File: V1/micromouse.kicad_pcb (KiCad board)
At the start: 2 copper layers, 98.1 x 98.9 mm, 22 parts, among them J1 XT60-M, SW1 SW_SPST, SW2 SW_Push, SW3 SW_SPDT_312, SW4 SW_Push, U1 BUCK, U10 UART, U2 STM32 Blackpill, U3 N20 encoder right, U4 N20 encoder left, U5 TB6612FNG, U6 VL6180X, U7 VL6180X, U8 VL6180X

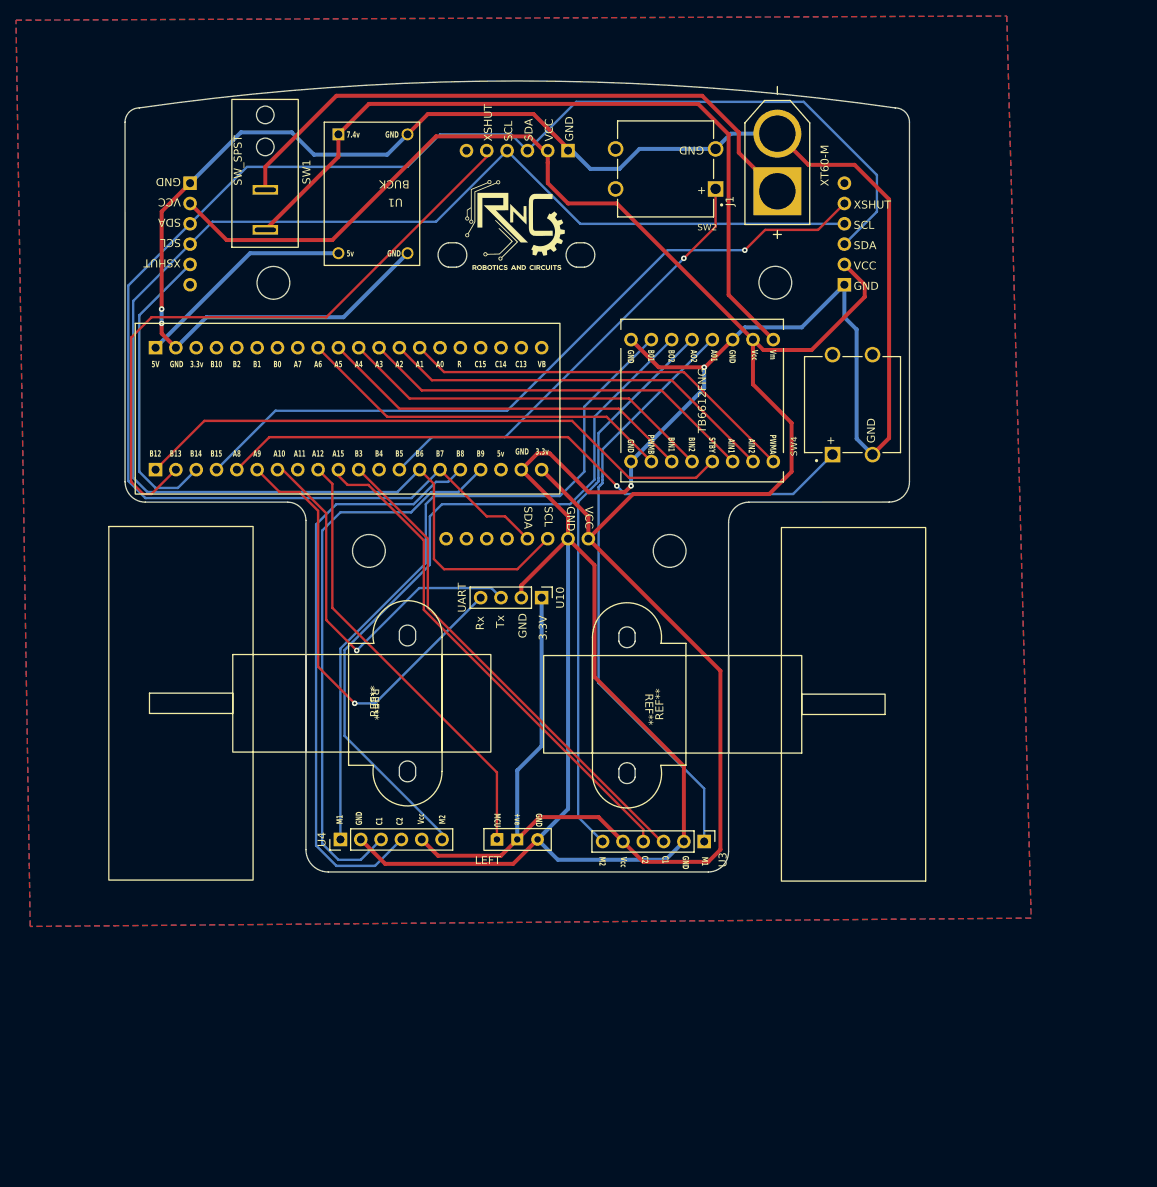
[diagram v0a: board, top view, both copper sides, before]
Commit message: v3 addition
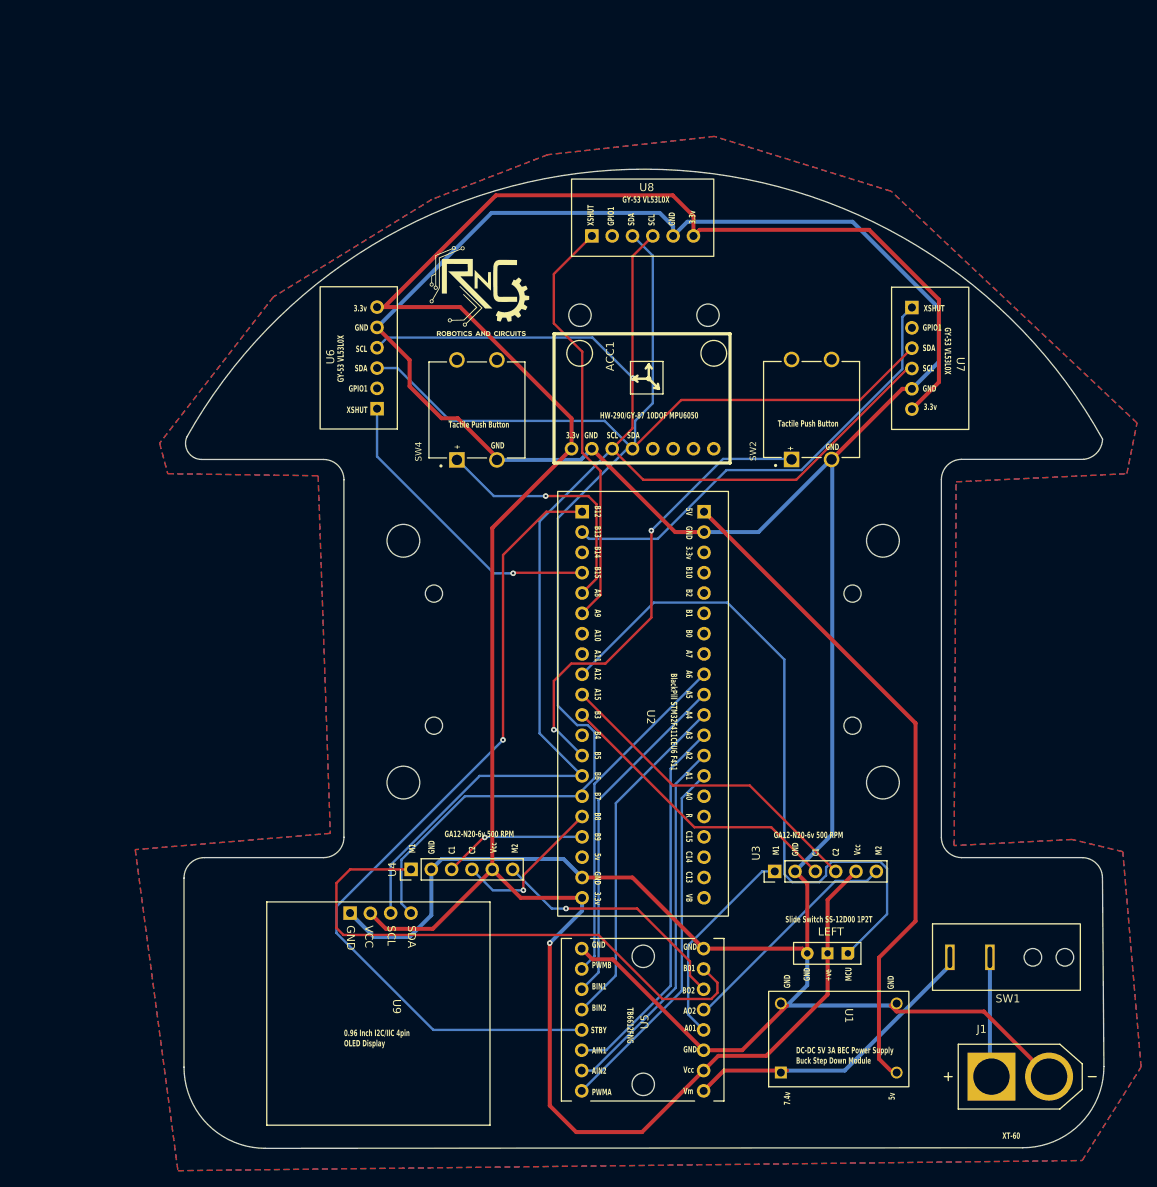
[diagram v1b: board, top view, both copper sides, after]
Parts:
- removed the G*** at (134.1, 40.9)
- removed the G*** at (134.1, 99.9)
- removed REF** (x2): n20 motor, n20 motor:n20 motor
- removed REF** (x2): n20 bracket, n20-bracket:Untitled
- removed REF**: castor, castor:castor
- removed U10: UART, Connector_PinHeader_2.54mm:PinHeader_1x04_P2.54mm_Vertical
- added G***: LOGO, rnc:rnc3, F.Cu at (129.7, 49.1)
- added U9: oled i2c, oled:oled, F.Cu at (118.5, 138.0)
- ACC1: moved to F.Cu
- U6: value VL6180X -> VL53L0X left; footprint VL6180X:VL6180X -> VL53L0X:VL53L0X; moved to F.Cu
- U7: value VL6180X -> VL53L0X right; footprint VL6180X:VL6180X -> VL53L0X:VL53L0X; moved to F.Cu
- U8: value VL6180X -> VL53L0X middle; footprint VL6180X:VL6180X -> VL53L0X:VL53L0X; moved to F.Cu
- moved SW1 135.0 mm to (195.4, 131.8), turned to 0 degrees
- moved U1 120.2 mm to (171.4, 140.6), turned to 90 degrees
- moved J1 118.2 mm to (197.0, 146.7), turned to 0 degrees
- moved U5 77.8 mm to (149.8, 139.6), turned to 180 degrees
- moved U6 55.8 mm to (119.1, 65.8)
- moved U7 48.2 mm to (180.9, 48.1), turned to -90 degrees
- moved SW4 47.0 mm to (129.1, 63.4)
- moved U8 42.1 mm to (140.9, 44.2), turned to 0 degrees
- moved SW3 39.7 mm to (173.0, 128.2), turned to 180 degrees
- moved ACC1 39.2 mm to (160.7, 70.0)
- moved SW2 35.2 mm to (170.9, 63.3), turned to 90 degrees
- moved U2 28.2 mm to (139.2, 73.6), turned to -90 degrees
- moved U3 9.58 mm to (166.3, 121.1), turned to 90 degrees
- moved U4 9.58 mm to (120.8, 120.8)
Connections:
- U2 pad 3: XSHUT 2 -> unconnected-(U2-B14-Pad3)
- U2 pad 6: Tx -> XSHUT 2
- U2 pad 7: Rx -> unconnected-(U2-A10-Pad7)
- U6 pad 1: unconnected-(U6-GPIO1-Pad1) -> 3.3v
- U6 pad 2: XSHUT 3 -> GND
- U6 pad 5: 3.3v -> unconnected-(U6-GPIO1-Pad5)
- U6 pad 6: GND -> XSHUT 3
- U7 pad 1: unconnected-(U7-GPIO1-Pad1) -> 3.3v
- U7 pad 2: XSHUT 1 -> GND
- U7 pad 5: 3.3v -> unconnected-(U7-GPIO1-Pad5)
- U7 pad 6: GND -> XSHUT 1
- U8 pad 1: unconnected-(U8-GPIO1-Pad1) -> 3.3v
- U8 pad 2: XSHUT 2 -> GND
- U8 pad 5: 3.3v -> unconnected-(U8-GPIO1-Pad5)
- U8 pad 6: GND -> XSHUT 2
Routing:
- net BO2: track 93.8 -> 31.1 mm, vias 0 -> 1
- net 7.4v: track 77.0 -> 15.0 mm
- net 7.4vb: track 95.6 -> 38.3 mm
- net Tx: track 56.9 -> 0.00 mm, vias 1 -> 0
- net 5v: track 27.8 -> 83.3 mm
- net XSHUT 3: track 92.3 -> 37.7 mm
- net encoder B2: track 74.1 -> 19.8 mm, vias 0 -> 1
- net encoder A2: track 71.3 -> 18.0 mm, vias 0 -> 1
- net push button: track 81.1 -> 31.5 mm
- net Rx: track 48.8 -> 0.00 mm, vias 1 -> 0
- net AO1: track 74.1 -> 26.0 mm
- net AO2: track 69.9 -> 28.7 mm
- net GND: track 430.2 -> 395.0 mm, vias 4 -> 0
- net slide_SW: track 55.5 -> 86.6 mm
- net STBY: track 75.9 -> 103.7 mm, vias 0 -> 1
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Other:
- board size 98.1 x 98.9 mm -> 115 x 122.4 mm
- board text added: "+"
- board text added: "+ve"
- board text added: "0.96 Inch I2C/IIC 4pin OLED Display"
- board text added: "3.3v"
- board text added: "5V"
- board text added: "5v"
- board text added: "7.4v"
- board text added: "A0"
- board text added: "A01"
- board text added: "A1"
- board text added: "A10"
- board text added: "A11"
- board text added: "A12"
- board text added: "A15"
- board text added: "A2"
- board text added: "A3"
- board text added: "A4"
- board text added: "A5"
- board text added: "A6"
- board text added: "A7"
- board text added: "A8"
- board text added: "A9"
- board text added: "AIN1"
- board text added: "AIN2"
- board text added: "AO2"
- board text added: "B0"
- board text added: "B01"
- board text added: "B1"
- board text added: "B10"
- board text added: "B12"
- board text added: "B13"
- board text added: "B14"
- board text added: "B15"
- board text added: "B2"
- board text added: "B3"
- board text added: "B4"
- board text added: "B5"
- board text added: "B6"
- board text added: "B7"
- board text added: "B8"
- board text added: "B9"
- board text added: "BIN1"
- board text added: "BIN2"
- board text added: "BO2"
- board text added: "BlackPill STM32F411CEU6 F411"
- board text added: "C1"
- board text added: "C13"
- board text added: "C14"
- board text added: "C15"
- board text added: "C2"
- board text added: "DC-DC 5V 3A BEC Power Supply Buck Step Down Module"
- board text added: "GA12-N20-6v 500 RPM"
- board text added: "GPIO1"
- board text added: "GY-53 VL53L0X"
- board text added: "HW-290/GY-87 10DOF MPU6050"
- board text added: "M1"
- board text added: "M2"
- board text added: "MCU"
- board text added: "PWMA"
- board text added: "PWMB"
- board text added: "R"
- board text added: "SCL"
- board text added: "SDA"
- board text added: "STBY"
- board text added: "Slide Switch SS-12D00 1P2T"
- board text added: "TB6612FNG"
- board text added: "Tactile Push Button"
- board text added: "VB"
- board text added: "Vcc"
- board text added: "Vm"
- board text added: "XSHUT"
- board text added: "XT-60"
- board text removed: "3.3V"
- board text removed: "Rx"
- board text removed: "Tx"
